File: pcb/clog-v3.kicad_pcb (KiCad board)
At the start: 2 copper layers, 125.3 x 81.8 mm, 32 parts, among them J0 AudioJack4dpb, SW1 SW_Push, SW10 SW_Push, SW11 SW_Push, SW12 SW_Push, SW13 SW_Push, SW14 SW_Push, SW15 SW_Push, SW16 SW_Push, SW17 SW_Push, SW18 SW_Push, SW19 SW_SPDT, SW2 SW_Push, SW20 SW_SPDT, SW21 SW_Push, SW3 SW_Push, SW4 SW_Push, SW5 SW_Push, SW6 SW_Push, SW7 SW_Push, SW8 SW_Push, SW9 SW_Push, U1 ProMicro_r

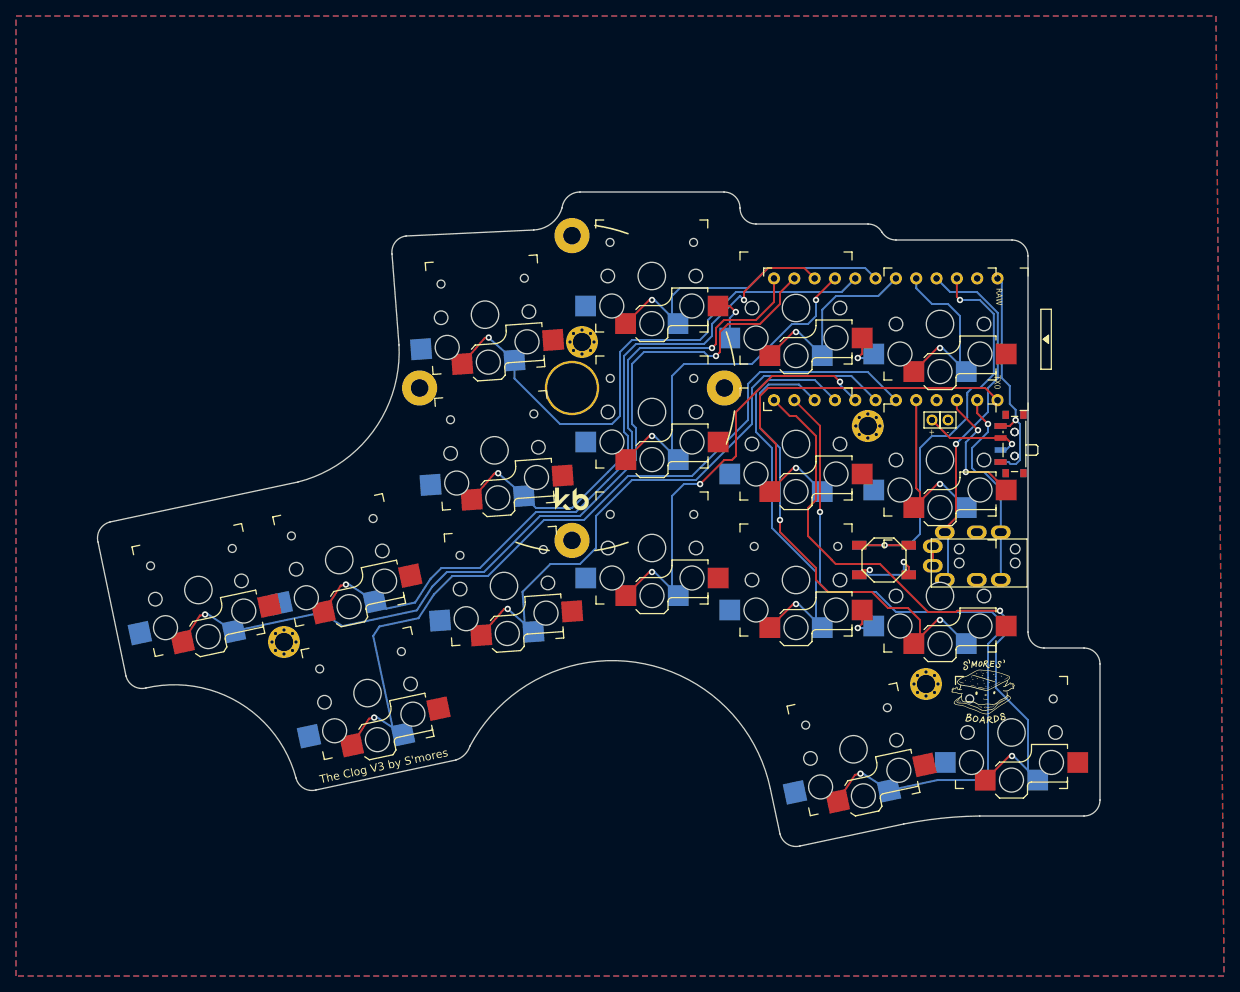
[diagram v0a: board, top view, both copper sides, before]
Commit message: Initial Case Work
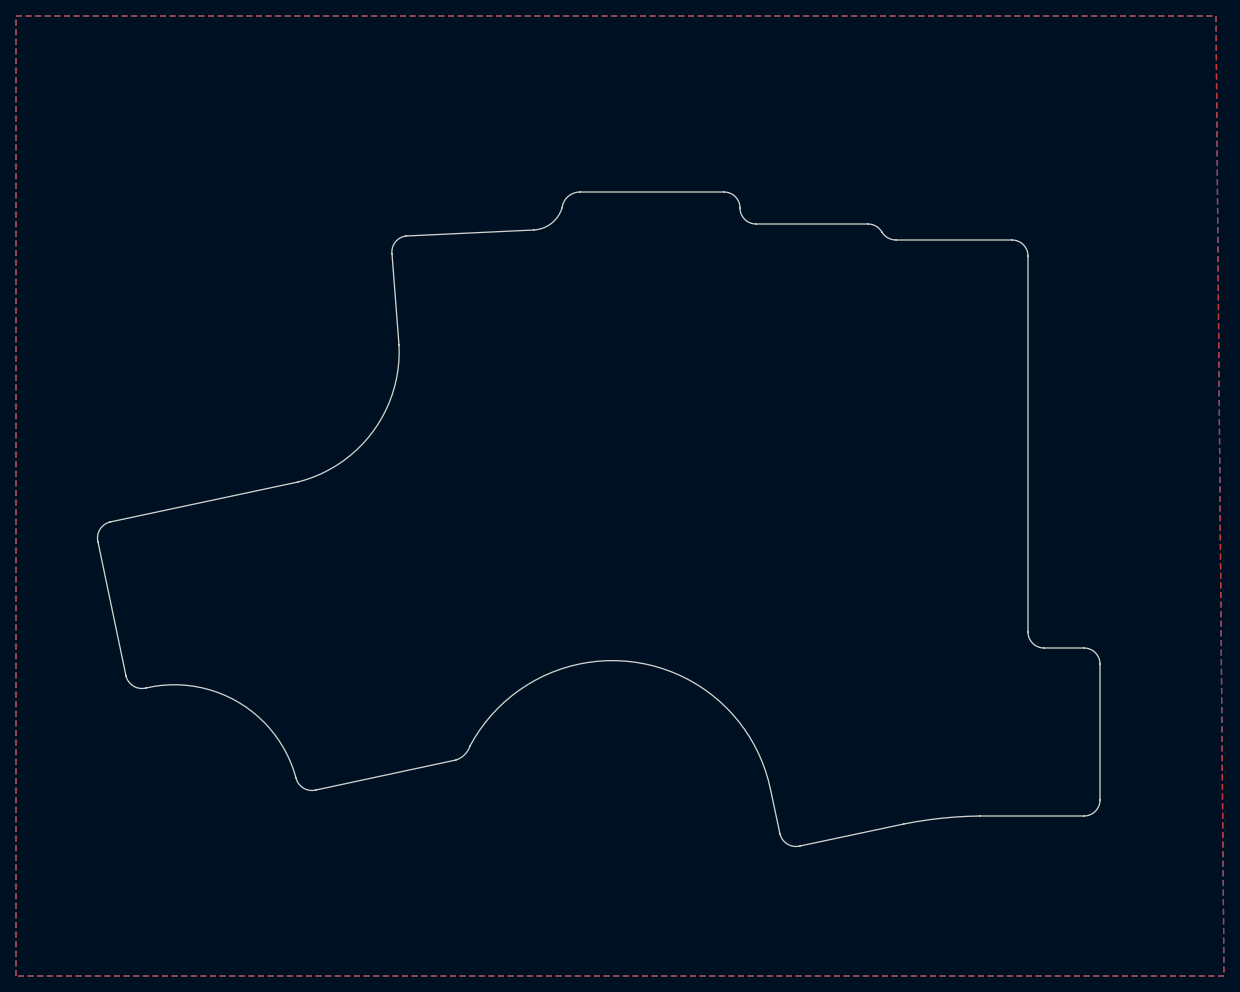
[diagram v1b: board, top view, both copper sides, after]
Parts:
- removed +1, -1: MountingHole_Pad, footprints:single-pin
- removed G*** (x2): LOGO, art:smores
- removed J0: AudioJack4dpb, footprints:trrs
- removed REF**: Tenting Puck, footprints:tenting-puck
- removed Ref** (x4): Val**, footprints:m2-hole
- removed SW1, SW10, SW11, SW12, SW13, SW14, SW15, SW16, SW17, SW2, SW3, SW4, SW5, SW6, SW7, SW8, SW9: SW_Push, footprints:choc-switch-socket-only
- removed SW18, SW21: SW_Push, footprints:reset-switch-4pin
- removed SW19, SW20: SW_SPDT, footprints:power-switch
- removed U1: ProMicro_r, footprints:pro-micro
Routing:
- net K5: track 107.9 -> 0.00 mm, vias 2 -> 0
- net K11: track 102.3 -> 0.00 mm, vias 1 -> 0
- net K16: track 90.4 -> 0.00 mm, vias 2 -> 0
- net K6: track 86.9 -> 0.00 mm, vias 2 -> 0
- net K17: track 81.4 -> 0.00 mm, vias 2 -> 0
- net K12: track 76.1 -> 0.00 mm, vias 1 -> 0
- net K1: track 69.4 -> 0.00 mm, vias 1 -> 0
- net K7: track 68.6 -> 0.00 mm, vias 2 -> 0
- net K15: track 61.7 -> 0.00 mm, vias 2 -> 0
- net K13: track 55.6 -> 0.00 mm, vias 3 -> 0
- net RESET: track 55.4 -> 0.00 mm, vias 2 -> 0
- net K14: track 53.4 -> 0.00 mm, vias 1 -> 0
- net K9: track 52.8 -> 0.00 mm, vias 1 -> 0
- net K8: track 46.6 -> 0.00 mm, vias 2 -> 0
- net VCC: track 45.9 -> 0.00 mm, vias 1 -> 0
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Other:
- board text removed: "+"
- board text removed: "-"
- board text removed: "RAW"
- board text removed: "The Clog V3 by S'mores"
